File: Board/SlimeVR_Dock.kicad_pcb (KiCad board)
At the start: 2 copper layers, 100 x 78.3 mm, 113 parts, among them J1Fan1 Conn_01x04_Pin, J1Temp1 Conn_01x05_Pin, J1_Control1 Conn_01x03_Pin, J1_MainPW1 USB_C_Receptacle_USB2.0_16P, J1_Monitor1 Conn_01x03_Pin, J1_Prog1 Conn_01x03_Pin, J2 USB_C_Receptacle_USB2.0_16P, J3 USB_C_Receptacle_USB2.0_16P, J4 USB_C_Receptacle_USB2.0_16P, J5 USB_C_Receptacle_USB2.0_16P, J6 USB_C_Receptacle_USB2.0_16P, J7 USB_C_Receptacle_USB2.0_16P, J8 USB_C_Receptacle_USB2.0_16P, J9 USB_C_Receptacle_USB2.0_16P, Q1 NDT452AP, Q2 BC857, Q3 BC857, Q4 BC857, Q5 BC857, Q6 BC817, U1 ESP32-C3-WROOM-02, U10 INA226, U11 AP22652W6-7, U12 INA226, U13 INA226, U14 AP22652W6-7, U15 INA226, U16 INA226, U17 74HC165, U18 74HC165, U19 74HC595, U2 CH224K, U3 XC6220B331MR, U4 TPS548A20RVER, U5 AP22652W6-7, U6 INA226, U7 INA226, U8 AP22652W6-7, U9 INA226

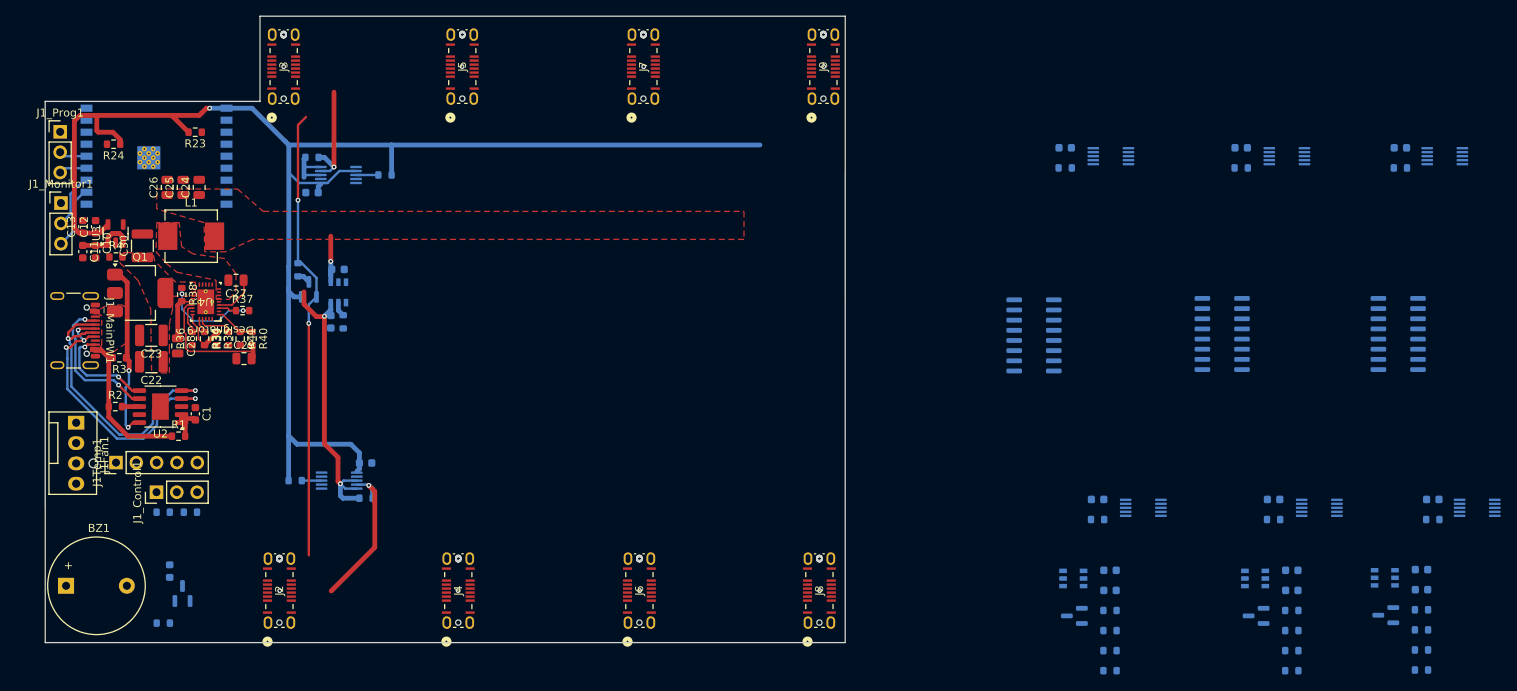
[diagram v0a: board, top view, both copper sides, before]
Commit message: almost finished layout V1
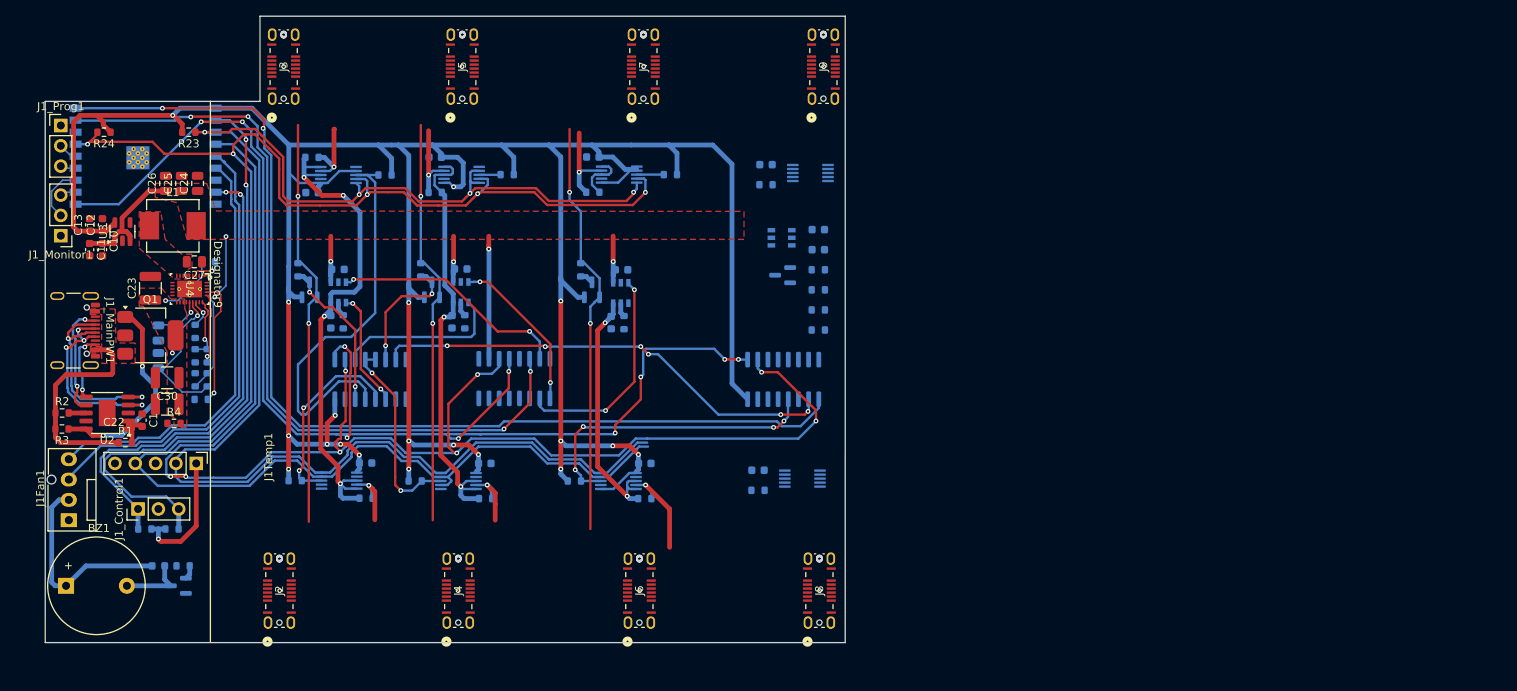
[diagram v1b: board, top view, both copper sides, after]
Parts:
- C28, C29, R34, R35, R36, R37, R38, R39, R40, R41: moved to B.Cu
- moved U17 128.6 mm to (136.7, 104.9), turned to -90 degrees
- moved R21 99.4 mm to (174.2, 79.3)
- moved R11 98.6 mm to (163.0, 91.2), turned to 90 degrees
- moved R20 97.6 mm to (153.8, 79.3)
- moved R8 96.1 mm to (143.0, 91.2), turned to 90 degrees
- moved Q4 92.5 mm to (164.4, 93.7), turned to 90 degrees
- moved R13 92.1 mm to (162.2, 117.6), turned to 0 degrees
- moved R12 91.9 mm to (168.4, 97.8), turned to -90 degrees
- moved C6 91.8 mm to (168.1, 91.2), turned to 0 degrees
- moved C7 91.4 mm to (166.8, 97.8), turned to -90 degrees
- moved Q3 90.0 mm to (144.4, 93.7), turned to 90 degrees
- moved C4 89.5 mm to (148.0, 91.1), turned to 0 degrees
- moved R9 89.4 mm to (148.5, 97.7), turned to -90 degrees
- moved R10 89.4 mm to (142.3, 117.6), turned to 0 degrees
- moved C5 88.8 mm to (146.9, 97.7), turned to -90 degrees
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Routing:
- net SDA: track 0.00 -> 222.4 mm, vias 0 -> 5
- net +3V3: track 189.8 -> 392.8 mm, vias 1 -> 20
- net SCL: track 0.00 -> 196.7 mm, vias 0 -> 4
- net CLK: track 0.00 -> 179.7 mm, vias 0 -> 8
- net GET: track 0.00 -> 162.7 mm, vias 0 -> 10
- net Data_Out: track 0.00 -> 131.8 mm, vias 0 -> 2
- net Data_In: track 0.00 -> 99.5 mm, vias 0 -> 4
- net 5VStepDwon: track 15.4 -> 93.8 mm, vias 1 -> 7
- net Enable: track 0.00 -> 73.6 mm, vias 0 -> 2
- net Boot: track 0.00 -> 60.6 mm, vias 0 -> 2
- net Net-(U17-~{Q7}): track 0.00 -> 58.3 mm, vias 0 -> 6
- net TACH: track 0.00 -> 57.3 mm
- net /Dual_USB-C_SubSchema1/USB_C0/VBUS: track 0.00 -> 53.9 mm, vias 0 -> 2
- net PWM: track 0.00 -> 53.7 mm
- net /Dual_USB-C_SubSchema2/USB_C0/CC_Line: track 0.00 -> 52.3 mm, vias 0 -> 2
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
